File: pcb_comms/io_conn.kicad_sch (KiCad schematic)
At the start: 10 parts, among them J1 Conn_01x06_Pin, J2 Conn_02x20_Odd_Even, J3 AUX2, J6 AUX1, J7 USB-B-Micro, J8 AUX2

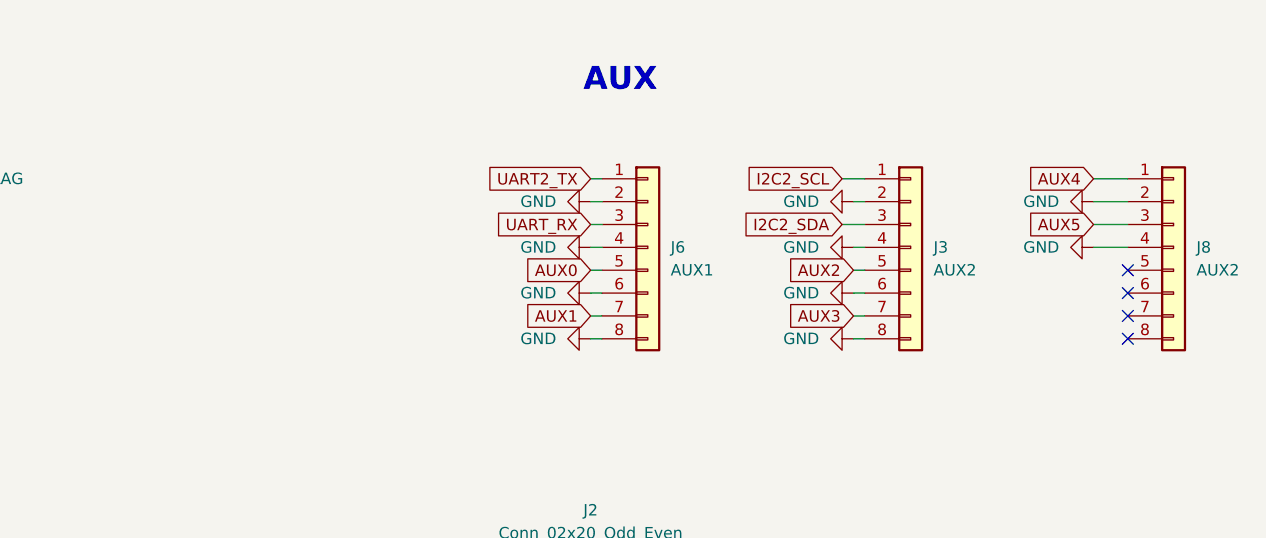
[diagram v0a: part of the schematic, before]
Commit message: Update route
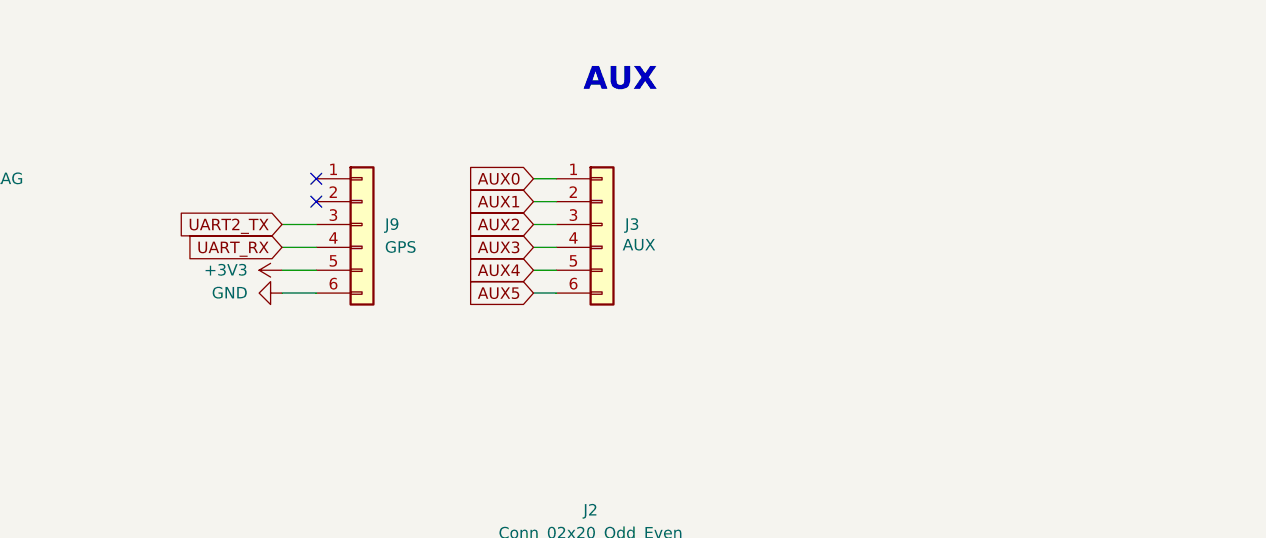
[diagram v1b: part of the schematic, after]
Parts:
- removed J3, J8: AUX2, Connector_PinSocket_2.54mm:PinSocket_1x08_P2.54mm_Vertical, symbol Connector_Generic:Conn_01x08
- removed J6: AUX1, Connector_PinSocket_2.54mm:PinSocket_1x08_P2.54mm_Vertical, symbol Connector_Generic:Conn_01x08
- added J3: AUX, JST B6B-XH-A-LF-SN-:CONN_B6B-XH-A_JST, symbol Connector_Generic:Conn_01x06
- added J9: GPS, Connector_JST:JST_SH_BM06B-SRSS-TB_1x06-1MP_P1.00mm_Vertical, symbol Connector_Generic:Conn_01x06
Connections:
- net +3V3: now also J9.5 (Pin_5)
- net AUX0: now also J3.1 (Pin_1)
- net AUX1: now also J3.2 (Pin_2)
- net AUX2: now also J3.3 (Pin_3)
- net AUX3: now also J3.4 (Pin_4)
- net AUX4: now also J3.5 (Pin_5)
- net AUX5: now also J3.6 (Pin_6)
- net GND: now also J9.6 (Pin_6)
- net UART2_TX: now also J9.3 (Pin_3)
- net UART_RX: now also J9.4 (Pin_4)
- no-connect marks 21 -> 19

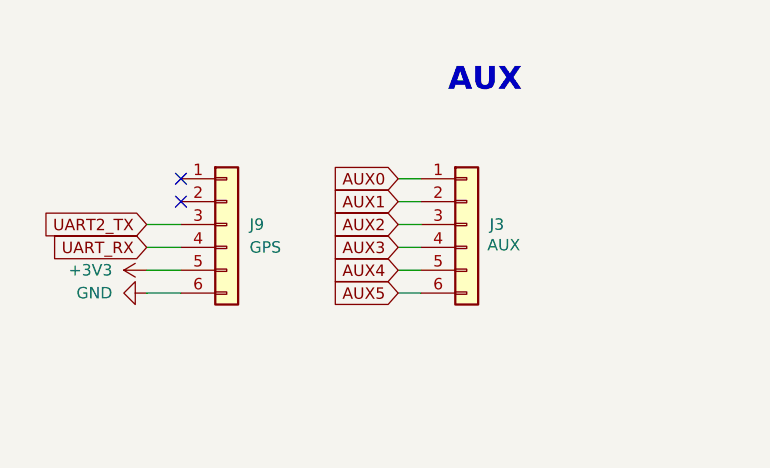
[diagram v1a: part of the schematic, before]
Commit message: Update schematic
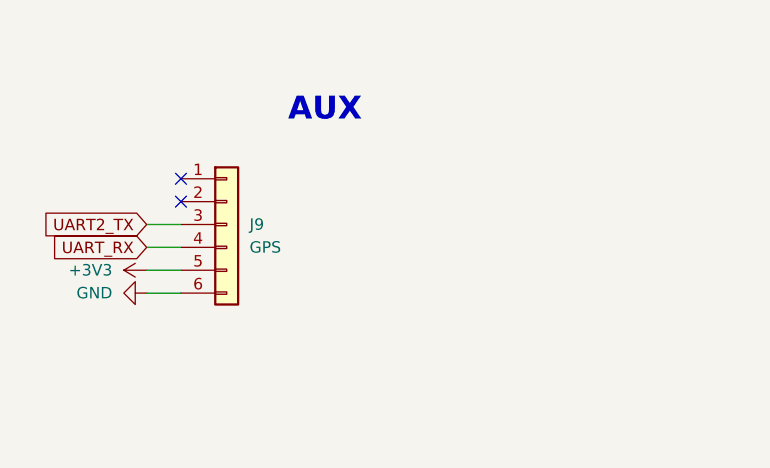
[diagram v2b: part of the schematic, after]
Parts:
- removed J3: AUX, JST B6B-XH-A-LF-SN-:CONN_B6B-XH-A_JST, symbol Connector_Generic:Conn_01x06

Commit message: PCB v2.1
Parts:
- J1: footprint Connector_PinHeader_2.54mm:PinHeader_1x06_P2.54mm_Vertical_SMD_Pin1Right -> CONN_01x06_87898-0666:CONN_01x06_87898-0666
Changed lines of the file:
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@@
+			)
+		)
+		(property "Sim.Device" ""
+			(at 43.18 97.79 0)
+			(effects
+				(font
+					(size 1.27 1.27)
+				)
+				(hide yes)
+			)
+		)
+		(property "Sim.Type" ""
+			(at 43.18 97.79 0)
+			(effects
+				(font
+					(size 1.27 1.27)
+				)
+				(hide yes)
 			)
 		)
@@
 			)
 		)
+		(property "Sim.Device" ""
+			(at 143.51 48.26 0)
+			(effects
+				(font
+					(size 1.27 1.27)
+				)
+				(hide yes)
+			)
+		)
+		(property "Sim.Type" ""
+			(at 143.51 48.26 0)
+			(effects
+				(font
+					(size 1.27 1.27)
+				)
+				(hide yes)
+			)
+		)
 		(pin "2"
 		)
@@
 			)
 		)
+		(property "Sim.Device" ""
+			(at 59.69 43.18 0)
+			(effects
+				(font
+					(size 1.27 1.27)
+				)
+				(hide yes)
+			)
+		)
+		(property "Sim.Type" ""
+			(at 59.69 43.18 0)
+			(effects
+				(font
+					(size 1.27 1.27)
+				)
+				(hide yes)
+			)
+		)
 		(pin "5"
 		)
@@
 			)
 		)
+		(property "Sim.Device" ""
+			(at 170.18 109.22 0)
+			(effects
+				(font
+					(size 1.27 1.27)
+				)
+				(hide yes)
+			)
+		)
+		(property "Sim.Type" ""
+			(at 170.18 109.22 0)
+			(effects
+				(font
+					(size 1.27 1.27)
+				)
+				(hide yes)
+			)
+		)
 		(pin "7"
 		)
@@
 			)
 		)
+		(property "Sim.Device" ""
+			(at 87.63 50.8 0)
+			(effects
+				(font
+					(size 1.27 1.27)
+				)
+				(hide yes)
+			)
+		)
+		(property "Sim.Type" ""
+			(at 87.63 50.8 0)
+			(effects
+				(font
+					(size 1.27 1.27)
+				)
+				(hide yes)
+			)
+		)
 		(pin "2"
 		)
@@
 			)
 		)
+		(property "Sim.Device" ""
+			(at 68.58 43.18 0)
+			(effects
+				(font
+					(size 1.27 1.27)
+				)
+				(hide yes)
+			)
+		)
+		(property "Sim.Type" ""
+			(at 68.58 43.18 0)
+			(effects
+				(font
+					(size 1.27 1.27)
+				)
+				(hide yes)
+			)
+		)
 		(pin "1"
 		)
@@
 			)
 		)
-		(property "Footprint" "Connector_PinHeader_2.54mm:PinHeader_1x06_P2.54mm_Vertical_SMD_Pin1Right"
+		(property "Footprint" "CONN_01x06_87898-0666:CONN_01x06_87898-0666"
 			(at 30.48 95.25 0)
 			(effects
@@
 		)
 		(property "KLC_S4.1" ""
+			(at 30.48 95.25 0)
+			(effects
+				(font
+					(size 1.27 1.27)
+				)
+				(hide yes)
+			)
+		)
+		(property "Sim.Device" ""
+			(at 30.48 95.25 0)
+			(effects
+				(font
+					(size 1.27 1.27)
+				)
+				(hide yes)
+			)
+		)
+		(property "Sim.Type" ""
 			(at 30.48 95.25 0)
 			(effects
@@
 			(at 74.93 102.87 0)
 			(effects
+				(font
+					(size 1.27 1.27)
+				)
+				(hide yes)
+			)
+		)
+		(property "Sim.Device" ""
+			(at 74.93 102.87 0)
+			(effects
+				(font
+					(size 1.27 1.27)
+				)
+				(hide yes)
+			)
+		)
+		(property "Sim.Type" ""
+			(at 74.93 102.87 0)
+			(effects
